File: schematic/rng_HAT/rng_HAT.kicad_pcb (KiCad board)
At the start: 2 copper layers, 56.5 x 65 mm, 32 parts, among them J1 RPi_GPIO, Q1 2N3904, Q2 2N3904, Q3 2N3904, Q4 BC107, Q5 2N3904, U3 STM32F103C8Tx

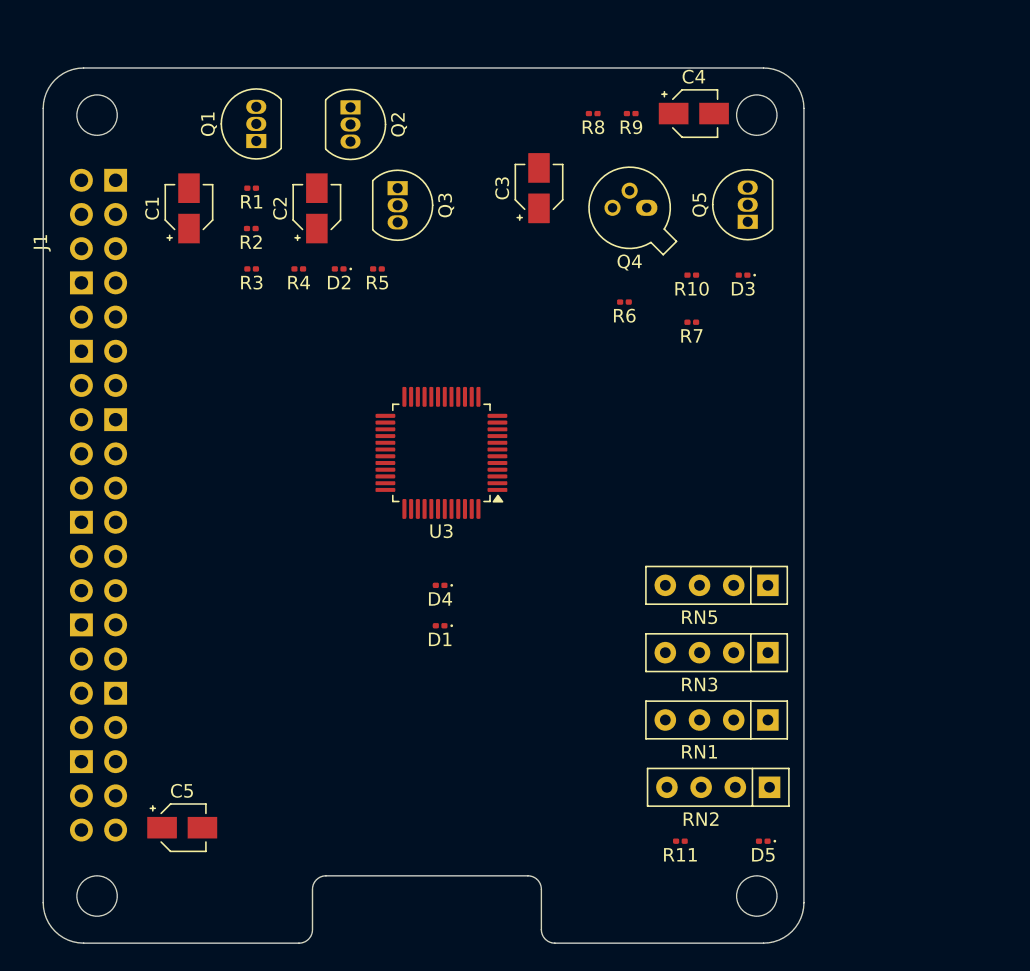
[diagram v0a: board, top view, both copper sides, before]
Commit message: some more PCB updates
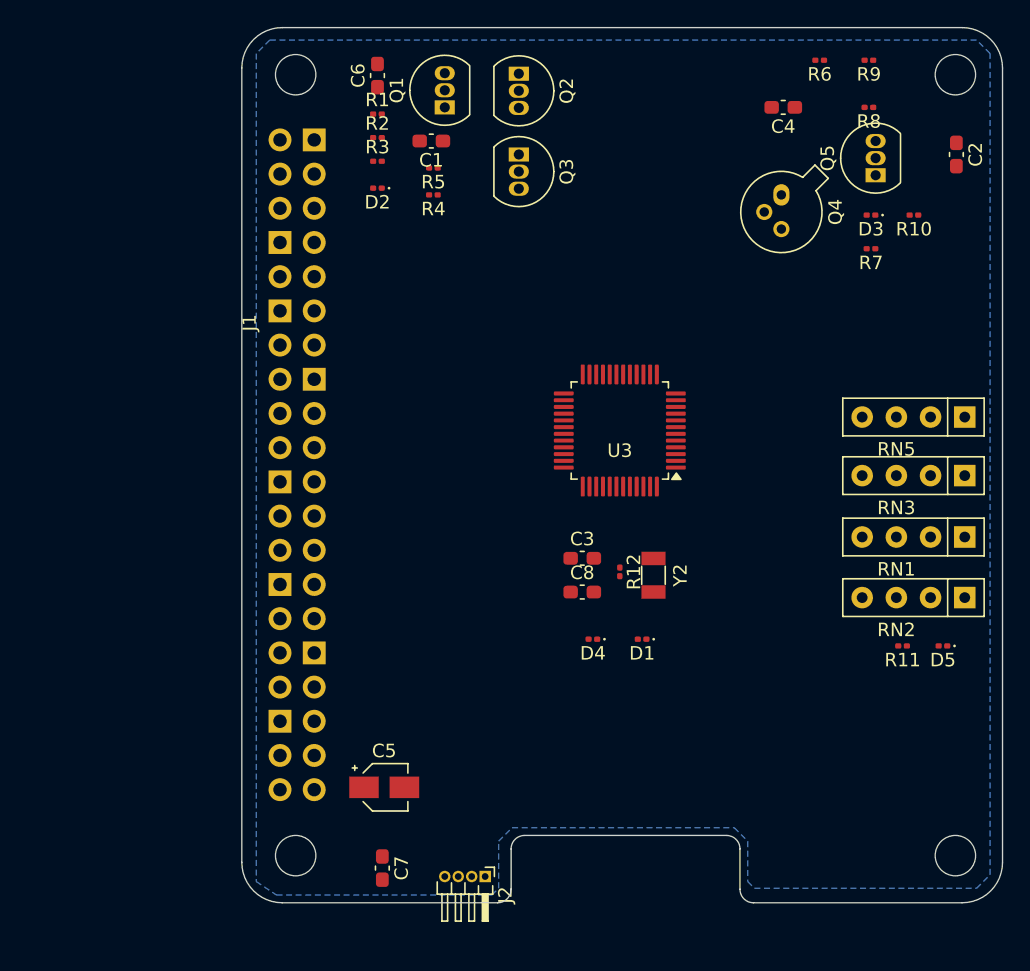
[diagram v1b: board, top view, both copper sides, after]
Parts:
- added C6: 10uF, Capacitor_SMD:C_0603_1608Metric_Pad1.08x0.95mm_HandSolder, F.Cu at (168.0, 86.1)
- added C7: 104nF, Capacitor_SMD:C_0603_1608Metric_Pad1.08x0.95mm_HandSolder, F.Cu at (168.4, 145.0)
- added C8: 20pF, Capacitor_SMD:C_0603_1608Metric_Pad1.08x0.95mm_HandSolder, F.Cu at (183.2, 124.5)
- added J2: Conn_01x04_Pin, Connector_PinHeader_1.00mm:PinHeader_1x04_P1.00mm_Horizontal, F.Cu at (176.0, 145.6)
- added R12: 1M, Resistor_SMD:R_0201_0603Metric, F.Cu at (186.0, 123.0)
- added Y2: 8MHz, Crystal:Crystal_SMD_3215-2Pin_3.2x1.5mm, F.Cu at (188.5, 123.2)
- C1: value 10uF -> 0.1uF; footprint Capacitor_SMD:CP_Elec_3x5.3 -> Capacitor_SMD:C_0603_1608Metric_Pad1.08x0.95mm_HandSolder
- C2: value 0.1uF -> 2.2uF; footprint Capacitor_SMD:CP_Elec_3x5.3 -> Capacitor_SMD:C_0603_1608Metric_Pad1.08x0.95mm_HandSolder
- C3: value 100nF -> 20pF; footprint Capacitor_SMD:CP_Elec_3x5.3 -> Capacitor_SMD:C_0603_1608Metric_Pad1.08x0.95mm_HandSolder
- C4: value 2.2uF -> 100nF; footprint Capacitor_SMD:CP_Elec_3x5.3 -> Capacitor_SMD:C_0603_1608Metric_Pad1.08x0.95mm_HandSolder
- D4: value GRN (FW ON) -> GRN (PWR ON)
- moved C2 47.7 mm to (211.0, 92.0), turned to -90 degrees
- moved C3 27.7 mm to (183.2, 122.0), turned to 0 degrees
- moved R6 23.1 mm to (200.8, 85.0)
- moved R11 22.0 mm to (207.0, 128.5)
- moved R8 20.5 mm to (204.5, 88.5)
- moved RN2 20.2 mm to (211.6, 124.9)
- moved RN1 20.0 mm to (211.6, 120.4)
- moved D5 19.7 mm to (210.0, 128.5)
- moved RN3 19.7 mm to (211.6, 115.8)
- moved RN5 19.2 mm to (211.6, 111.5)
- moved C1 18.7 mm to (172.0, 91.0), turned to 180 degrees
- moved R9 18.1 mm to (204.5, 85.0)
- moved R10 17.1 mm to (207.8, 96.5)
- moved C5 15.3 mm to (168.5, 139.0)
- moved J1 15.1 mm to (161.9, 115.1)
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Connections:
- C1 pad 1: 5V -> Net-(Q1-E)
- C1 pad 2: GND -> Net-(Q3-B)
- C2 pad 1: Net-(Q3-B) -> Net-(Q5-C)
- C2 pad 2: Net-(Q1-E) -> WN OUT
- C3 pad 1: Net-(Q4-C) -> GND
- C3 pad 2: Net-(Q5-B) -> Net-(U3-PD1)
- C4 pad 1: Net-(Q5-C) -> Net-(Q4-C)
- C4 pad 2: WN OUT -> Net-(Q5-B)
- U3 pad 34: unconnected-(U3-PA13-Pad34) -> Net-(J2-Pin_2)
- U3 pad 37: unconnected-(U3-PA14-Pad37) -> Net-(J2-Pin_3)
- U3 pad 5: unconnected-(U3-PD0-Pad5) -> Net-(U3-PD0)
- U3 pad 6: unconnected-(U3-PD1-Pad6) -> Net-(U3-PD1)
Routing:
- added copper zone on B.Cu, net GND
